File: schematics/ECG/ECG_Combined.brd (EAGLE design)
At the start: 25.4 x 25.4 mm, 73 parts, among them IC1 ADS1293, IC2 LIS3DH, IC3 MCP1703, IC4 CC2541, IC5 FSA4157, IC6 FSA4157, IC7 FSA4157, X1 XTAL-2SMD, X2 XTAL_403, X3 XTAL-CSM7

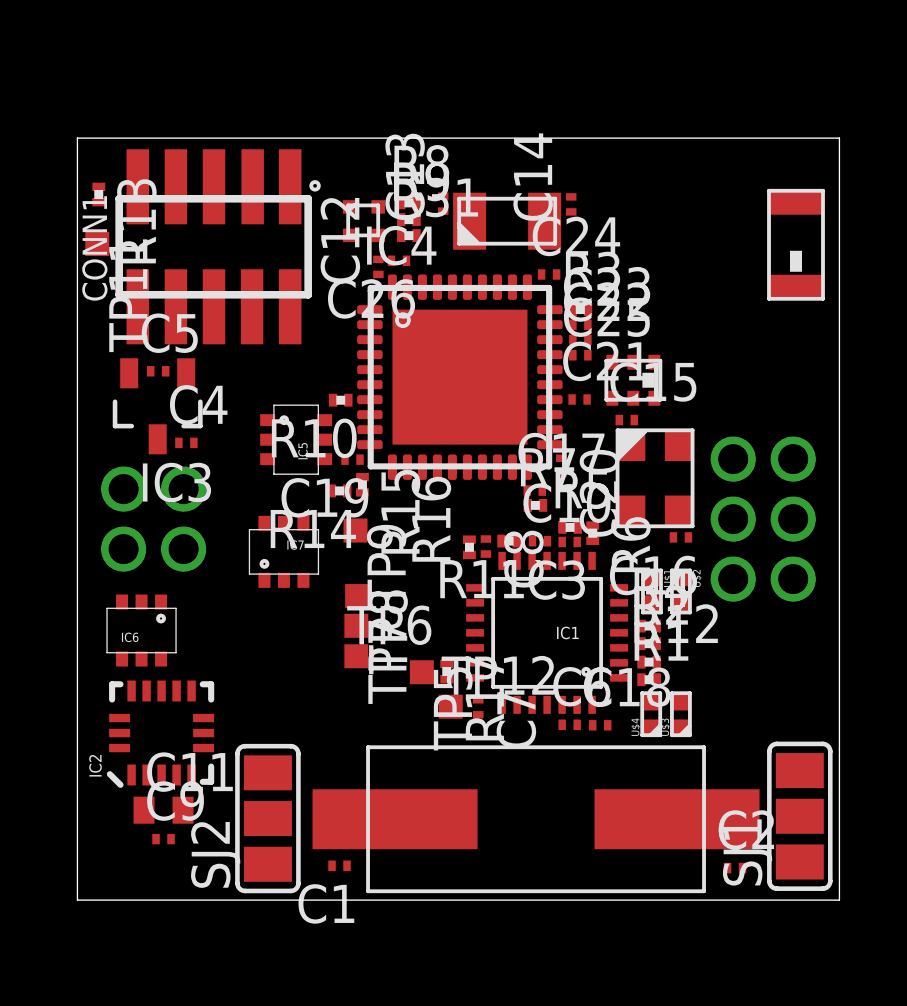
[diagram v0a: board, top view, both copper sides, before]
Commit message: continued routing
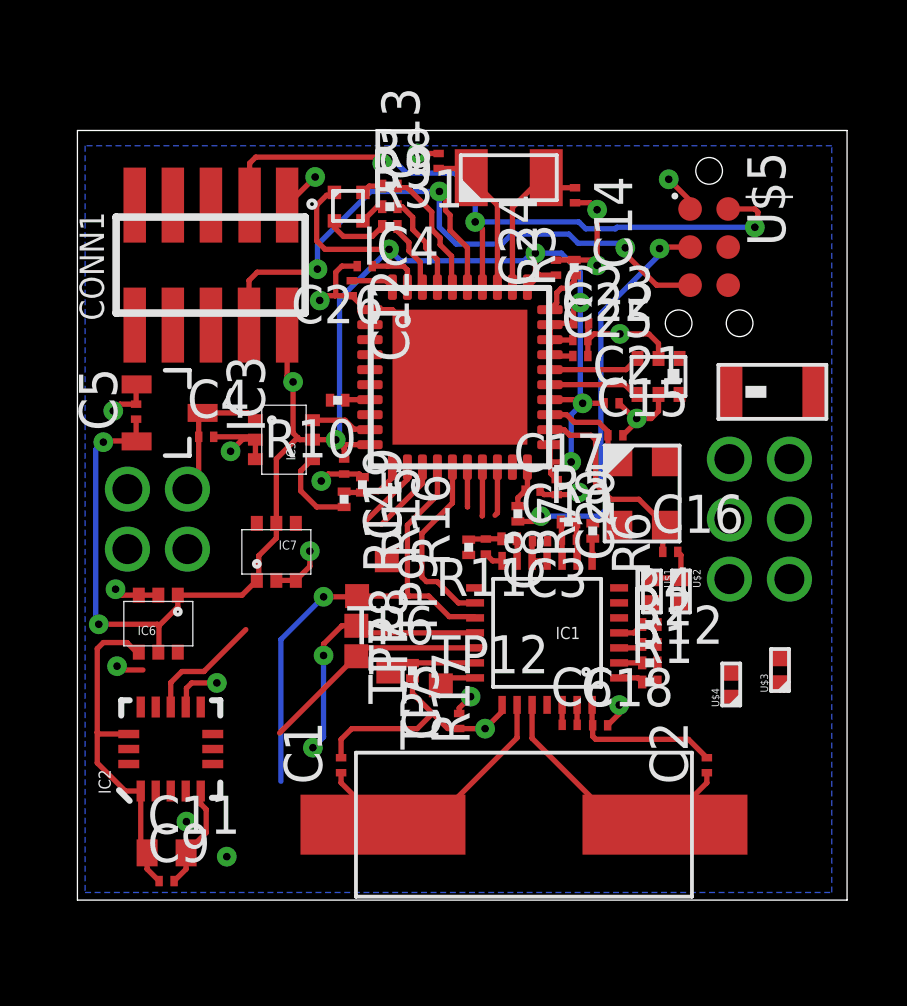
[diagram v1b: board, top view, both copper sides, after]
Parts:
- removed R13: 0, rcl:R0201
- removed SJ1, SJ2: (no value), jumper:SJ_2
- removed TP11: TPSTP08SQ, testpad:TP08SQ
- added U$5: TC2030-MCP-NL, tagconnect:TC2030-MCP-NL
- moved RF 5.03 mm to (23.2, 16.9), turned to 180 degrees
- moved U$3 3.62 mm to (23.4, 7.67)
- moved C2 3.56 mm to (21.0, 4.50), turned to 90 degrees
- moved C1 3.35 mm to (8.79, 4.50), turned to 90 degrees
- moved U$4 2.85 mm to (21.8, 7.19)
- moved C5 1.53 mm to (1.96, 16.3), turned to 90 degrees
- moved X1 1.45 mm to (14.4, 24.1)
- moved TP9 1.44 mm to (10.3, 11.3)
- moved C13 1.43 mm to (12.0, 24.6)
- moved C11 1.43 mm to (2.97, 1.57)
- moved R3 1.41 mm to (16.6, 21.1), turned to 90 degrees
- moved C9 1.40 mm to (2.97, 0.64)
- moved C26 1.16 mm to (9.58, 21.1)
- moved R17 1.14 mm to (11.2, 7.64)
- moved C12 1.14 mm to (9.14, 20.4), turned to 270 degrees
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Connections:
- removed net N$1: CONN1.9, R13.1
- removed net N$10: C2.2, SJ1.2
- removed net N$13: C1.2, SJ2.2
- removed net N$2: R13.2, TP11.TP
- net ECG_VCC: now also C1.2, C2.2
- net GND: now also U$5.1; no longer SJ1.3, SJ2.3
- net P2_1/DD: now also U$5.5
- net P2_2/DC: now also U$5.2
- net RESET_N: now also U$5.3
- net VCC: now also U$5.4; no longer SJ1.1, SJ2.1
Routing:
- net VCC: track 0.00 -> 64.9 mm, vias 0 -> 9
- net GND: track 0.00 -> 43.8 mm, vias 0 -> 19
- net P2_1/DD: track 0.00 -> 23.9 mm, vias 0 -> 3
- net P2_2/DC: track 0.00 -> 23.7 mm, vias 0 -> 3
- net SPI_CLK: track 0.00 -> 16.8 mm, vias 0 -> 2
- net ECG_VCC: track 0.00 -> 14.7 mm, vias 0 -> 1
- net RESET_N: track 0.00 -> 13.7 mm, vias 0 -> 2
- net ACCEL_VCC: track 0.00 -> 11.6 mm
- net SPI_MOSI: track 0.00 -> 10.3 mm, vias 0 -> 2
- net SPI_MISO: track 0.00 -> 9.33 mm
- net XTAL1: track 0.00 -> 9.08 mm
- net XTAL2: track 0.00 -> 9.05 mm
- net XOSC_Q2: track 0.00 -> 6.94 mm
- net ACCEL_INT1: track 0.00 -> 6.52 mm
- net SPI_SS: track 0.00 -> 6.22 mm
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- added copper zone on layer 16, net GND
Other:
- board size 25.4 x 25.4 mm -> 25.7 x 25.7 mm
